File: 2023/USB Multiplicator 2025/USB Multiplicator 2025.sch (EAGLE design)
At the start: 11 parts, among them X1 USB-A

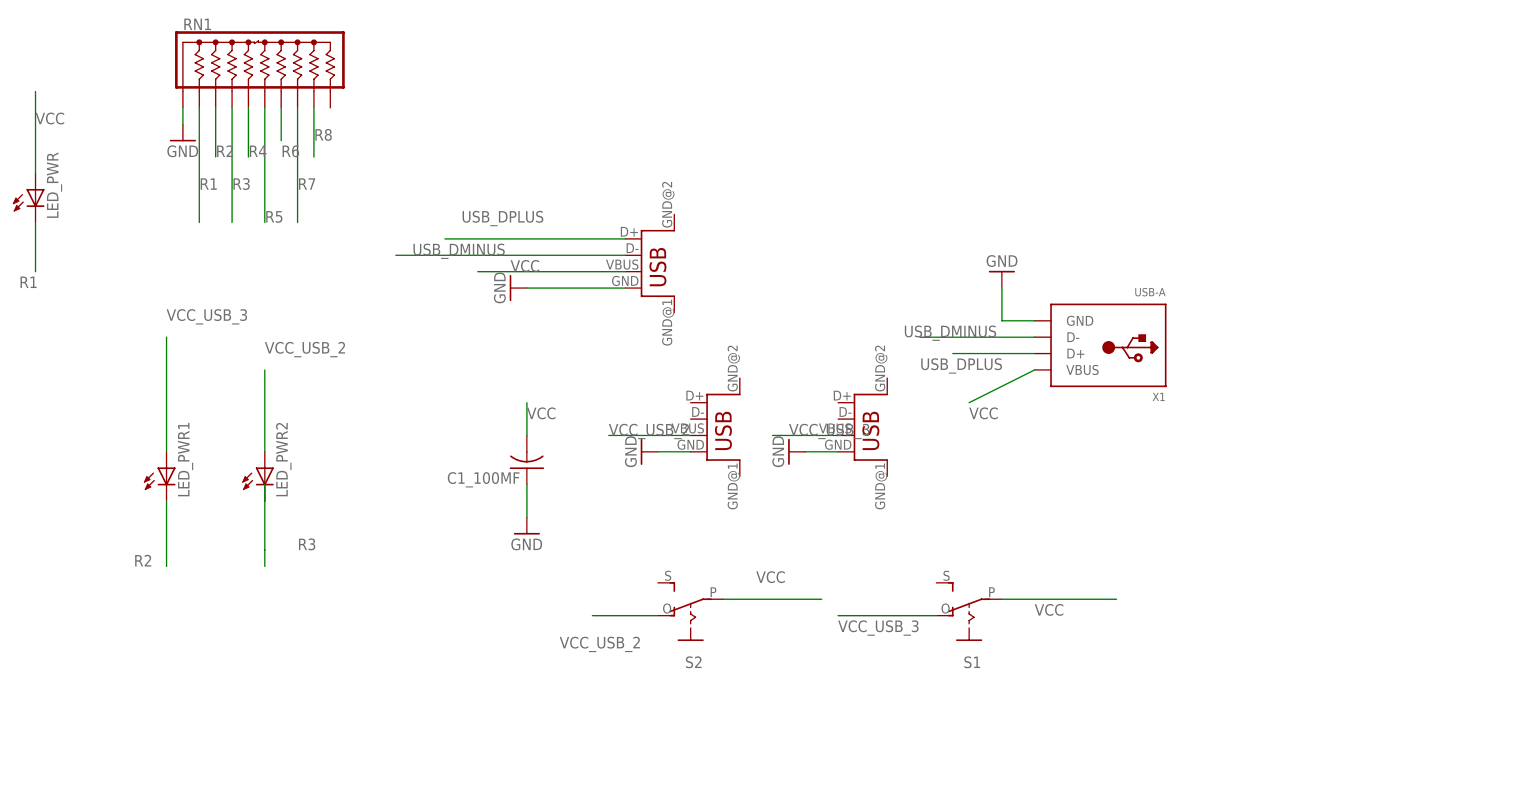
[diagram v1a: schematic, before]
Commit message: Update...
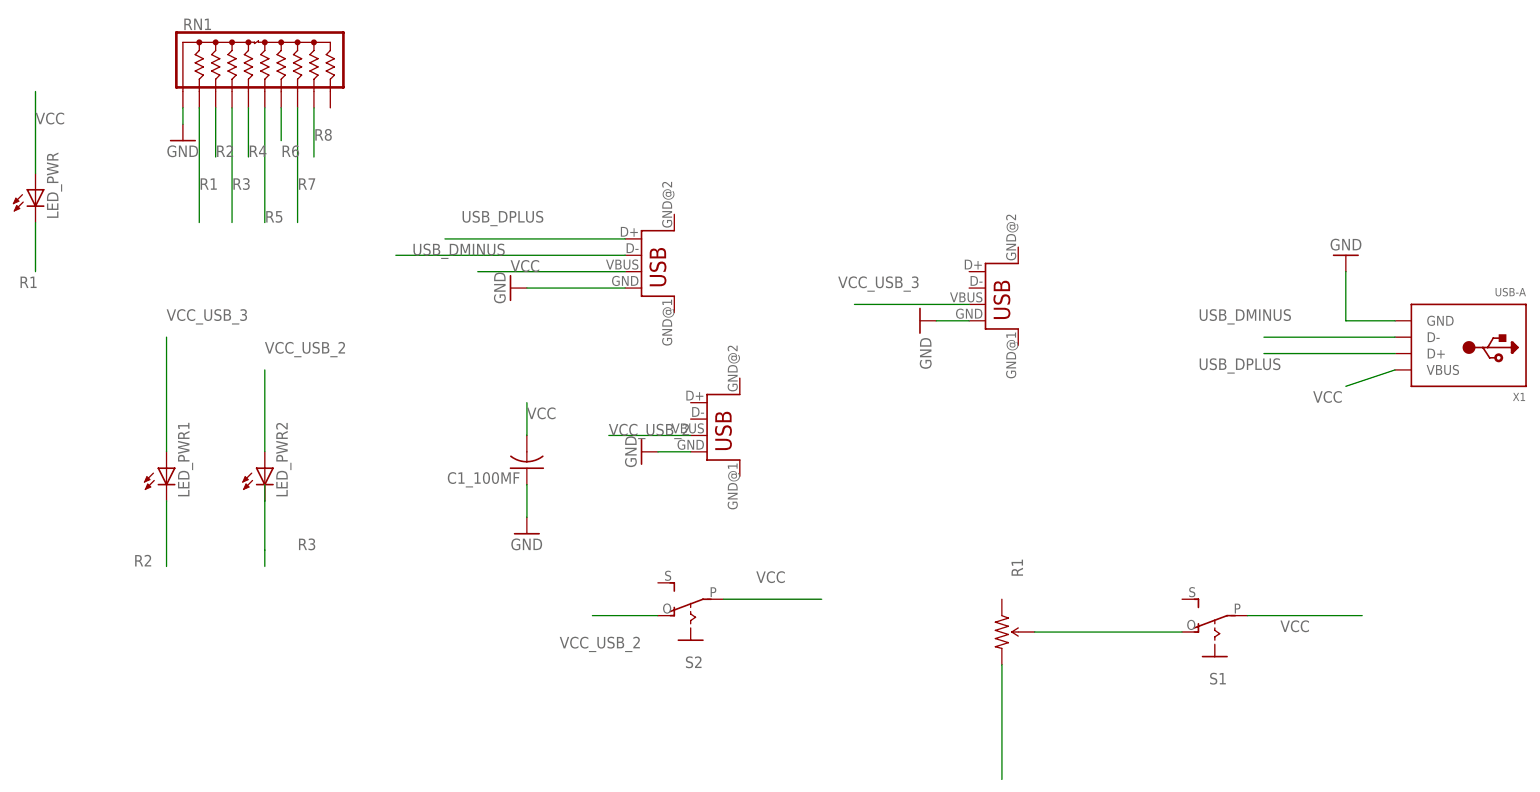
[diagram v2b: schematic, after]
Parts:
- added R1: (no value), SparkFun-Retired:TRIMPOTPTH
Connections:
- new net N$1: R1.WIPER, S1.O
- net VCC_USB_3: now also R1.CW; no longer S1.O
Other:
- moved on the sheet: S1, X1
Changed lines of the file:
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@@
 <layer number="56" name="wert" color="7" fill="1" visible="no" active="no"/>
 <layer number="57" name="tCAD" color="7" fill="1" visible="no" active="no"/>
+<layer number="59" name="tCarbon" color="7" fill="1" visible="no" active="no"/>
+<layer number="60" name="bCarbon" color="7" fill="1" visible="no" active="no"/>
+<layer number="88" name="SimResults" color="9" fill="1" visible="yes" active="yes"/>
+<layer number="89" name="SimProbes" color="9" fill="1" visible="yes" active="yes"/>
 <layer number="90" name="Modules" color="5" fill="1" visible="yes" active="yes"/>
 <layer number="91" name="Nets" color="2" fill="1" visible="yes" active="yes"/>
@@
 <layer number="112" name="tSilk" color="7" fill="1" visible="no" active="yes"/>
 <layer number="113" name="ReferenceLS" color="7" fill="1" visible="no" active="no"/>
+<layer number="114" name="Badge_Outline" color="11" fill="1" visible="no" active="no"/>
+<layer number="115" name="ReferenceISLANDS" color="7" fill="1" visible="yes" active="yes"/>
 <layer number="116" name="Patch_BOT" color="9" fill="4" visible="no" active="yes"/>
 <layer number="118" name="Rect_Pads" color="7" fill="1" visible="no" active="no"/>
@@
 <layer number="127" name="_tValues" color="7" fill="1" visible="no" active="yes"/>
 <layer number="128" name="_bValues" color="7" fill="1" visible="no" active="yes"/>
+<layer number="129" name="Mask" color="7" fill="1" visible="yes" active="yes"/>
 <layer number="131" name="tAdjust" color="7" fill="1" visible="no" active="yes"/>
 <layer number="132" name="bAdjust" color="7" fill="1" visible="no" active="yes"/>
@@
 <layer number="251" name="SMDround" color="7" fill="1" visible="no" active="no"/>
 <layer number="254" name="cooling" color="7" fill="1" visible="no" active="yes"/>
+<layer number="255" name="routoute" color="7" fill="1" visible="yes" active="yes"/>
 </layers>
 <schematic xreflabel="%F%N/%S.%C%R" xrefpart="/%S.%C%R">
@@
 <part name="RN1" library="resistor-sip" deviceset="4610X" device=""/>
 <part name="GND9" library="supply1" deviceset="GND" device=""/>
+<part name="R1" library="SparkFun-Retired" deviceset="TRIMPOT" device="PTH"/>
 </parts>
 <sheets>
@@
 </plain>
 <instances>
-<instance part="X1" gate="G$1" x="127" y="99.06" smashed="yes" rot="R180">
-<attribute name="NAME" x="137.16" y="90.424" size="1.27" layer="95" rot="R180"/>
-<attribute name="VALUE" x="137.16" y="106.68" size="1.27" layer="96" rot="R180"/>
-</instance>
-<instance part="GND1" gate="1" x="111.76" y="109.22" smashed="yes" rot="R180">
-<attribute name="VALUE" x="114.3" y="111.76" size="1.778" layer="96" rot="R180"/>
+<instance part="X1" gate="G$1" x="182.88" y="99.06" smashed="yes" rot="R180">
+<attribute name="NAME" x="193.04" y="90.424" size="1.27" layer="95" rot="R180"/>
+<attribute name="VALUE" x="193.04" y="106.68" size="1.27" layer="96" rot="R180"/>
+</instance>
+<instance part="GND1" gate="1" x="165.1" y="111.76" smashed="yes" rot="R180">
+<attribute name="VALUE" x="167.64" y="114.3" size="1.778" layer="96" rot="R180"/>
 </instance>
 <instance part="C1_100MF" gate="G$1" x="38.1" y="78.74" smashed="yes" rot="R180">
@@
 </instance>
 <instance part="USB_OUT_2" gate="G$1" x="66.04" y="78.74" smashed="yes"/>
-<instance part="USB_OUT_3" gate="G$1" x="88.9" y="78.74" smashed="yes"/>
+<instance part="USB_OUT_3" gate="G$1" x="109.22" y="99.06" smashed="yes"/>
 <instance part="GND3" gate="1" x="55.88" y="81.28" smashed="yes" rot="R270">
 <attribute name="VALUE" x="53.34" y="83.82" size="1.778" layer="96" rot="R270"/>
 </instance>
-<instance part="GND4" gate="1" x="78.74" y="81.28" smashed="yes" rot="R270">
-<attribute name="VALUE" x="76.2" y="83.82" size="1.778" layer="96" rot="R270"/>
+<instance part="GND4" gate="1" x="99.06" y="101.6" smashed="yes" rot="R270">
+<attribute name="VALUE" x="99.06" y="99.06" size="1.778" layer="96" rot="R270"/>
 </instance>
 <instance part="S2" gate="1" x="63.5" y="55.88" smashed="yes" rot="R90">
@@
 <attribute name="VALUE" x="60.325" y="52.07" size="1.778" layer="96" rot="R180"/>
 </instance>
-<instance part="S1" gate="1" x="106.68" y="55.88" smashed="yes" rot="R90">
-<attribute name="NAME" x="108.585" y="49.53" size="1.778" layer="95" rot="R180"/>
-<attribute name="VALUE" x="103.505" y="52.07" size="1.778" layer="96" rot="R180"/>
+<instance part="S1" gate="1" x="144.78" y="53.34" smashed="yes" rot="R90">
+<attribute name="NAME" x="146.685" y="46.99" size="1.778" layer="95" rot="R180"/>
+<attribute name="VALUE" x="141.605" y="49.53" size="1.778" layer="96" rot="R180"/>
 </instance>
 <instance part="LED_PWR2" gate="G$1" x="-2.54" y="78.74" smashed="yes">
@@
 <instance part="GND9" gate="1" x="-15.24" y="129.54" smashed="yes">
 <attribute name="VALUE" x="-17.78" y="127" size="1.778" layer="96"/>
+</instance>
+<instance part="R1" gate="R?" x="111.76" y="53.34" smashed="yes" rot="R270">
+<attribute name="NAME" x="113.2586" y="64.77" size="1.778" layer="95" rot="R270"/>
+<attribute name="VALUE" x="108.458" y="57.15" size="1.778" layer="96" rot="R270"/>
 </instance>
 </instances>
@@
 <segment>
 <pinref part="X1" gate="G$1" pin="GND"/>
-<wire x1="116.84" y1="101.6" x2="111.76" y2="101.6" width="0.1524" layer="91"/>
+<wire x1="172.72" y1="101.6" x2="165.1" y2="101.6" width="0.1524" layer="91"/>
 <pinref part="GND1" gate="1" pin="GND"/>
-<wire x1="111.76" y1="101.6" x2="111.76" y2="106.68" width="0.1524" layer="91"/>
+<wire x1="165.1" y1="101.6" x2="165.1" y2="109.22" width="0.1524" layer="91"/>
 </segment>
 <segment>
@@
 <pinref part="GND4" gate="1" pin="GND"/>
 <pinref part="USB_OUT_3" gate="G$1" pin="GND"/>
-<wire x1="81.28" y1="81.28" x2="86.36" y2="81.28" width="0.1524" layer="91"/>
+<wire x1="101.6" y1="101.6" x2="106.68" y2="101.6" width="0.1524" layer="91"/>
 </segment>
 <segment>
@@
 <segment>
 <pinref part="X1" gate="G$1" pin="VBUS"/>
-<wire x1="116.84" y1="93.98" x2="106.68" y2="88.9" width="0.1524" layer="91"/>
-<label x="106.68" y="86.36" size="1.778" layer="95"/>
+<wire x1="172.72" y1="93.98" x2="165.1" y2="91.44" width="0.1524" layer="91"/>
+<label x="160.02" y="88.9" size="1.778" layer="95"/>
 </segment>
 <segment>
 <pinref part="S1" gate="1" pin="P"/>
-<wire x1="111.76" y1="58.42" x2="129.54" y2="58.42" width="0.1524" layer="91"/>
-<label x="116.84" y="55.88" size="1.778" layer="95"/>
+<wire x1="149.86" y1="55.88" x2="167.64" y2="55.88" width="0.1524" layer="91"/>
+<label x="154.94" y="53.34" size="1.778" layer="95"/>
 </segment>
 </net>
@@
 <segment>
 <pinref part="X1" gate="G$1" pin="D+"/>
-<wire x1="116.84" y1="96.52" x2="104.14" y2="96.52" width="0.1524" layer="91"/>
-<label x="99.06" y="93.98" size="1.778" layer="95"/>
+<wire x1="172.72" y1="96.52" x2="152.4" y2="96.52" width="0.1524" layer="91"/>
+<label x="142.24" y="93.98" size="1.778" layer="95"/>
 </segment>
 <segment>
@@
 <segment>
 <pinref part="X1" gate="G$1" pin="D-"/>
-<wire x1="116.84" y1="99.06" x2="99.06" y2="99.06" width="0.1524" layer="91"/>
-<label x="96.52" y="99.06" size="1.778" layer="95"/>
+<wire x1="172.72" y1="99.06" x2="152.4" y2="99.06" width="0.1524" layer="91"/>
+<label x="142.24" y="101.6" size="1.778" layer="95"/>
 </segment>
 <segment>
@@
 <segment>
 <pinref part="USB_OUT_3" gate="G$1" pin="VBUS"/>
-<wire x1="86.36" y1="83.82" x2="76.2" y2="83.82" width="0.1524" layer="91"/>
-<label x="78.74" y="83.82" size="1.778" layer="95"/>
-</segment>
-<segment>
-<pinref part="S1" gate="1" pin="O"/>
-<wire x1="101.6" y1="55.88" x2="86.36" y2="55.88" width="0.1524" layer="91"/>
-<label x="86.36" y="53.34" size="1.778" layer="95"/>
+<wire x1="106.68" y1="104.14" x2="88.9" y2="104.14" width="0.1524" layer="91"/>
+<label x="86.36" y="106.68" size="1.778" layer="95"/>
 </segment>
 <segment>
@@
 <wire x1="-17.78" y1="81.28" x2="-17.78" y2="99.06" width="0.1524" layer="91"/>
 <label x="-17.78" y="101.6" size="1.778" layer="95"/>
+</segment>
+<segment>
+<pinref part="R1" gate="R?" pin="CW"/>
+<wire x1="111.76" y1="48.26" x2="111.76" y2="30.48" width="0.1524" layer="91"/>
 </segment>
 </net>
@@
 </segment>
 </net>
+<net name="N$1" class="0">
+<segment>
+<pinref part="S1" gate="1" pin="O"/>
+<pinref part="R1" gate="R?" pin="WIPER"/>
+<wire x1="139.7" y1="53.34" x2="116.84" y2="53.34" width="0.1524" layer="91"/>
+</segment>
+</net>

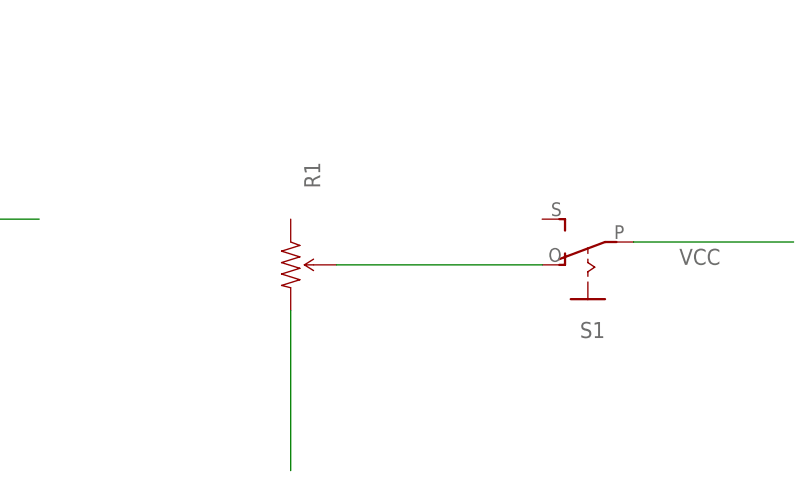
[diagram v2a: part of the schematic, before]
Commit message: Update...
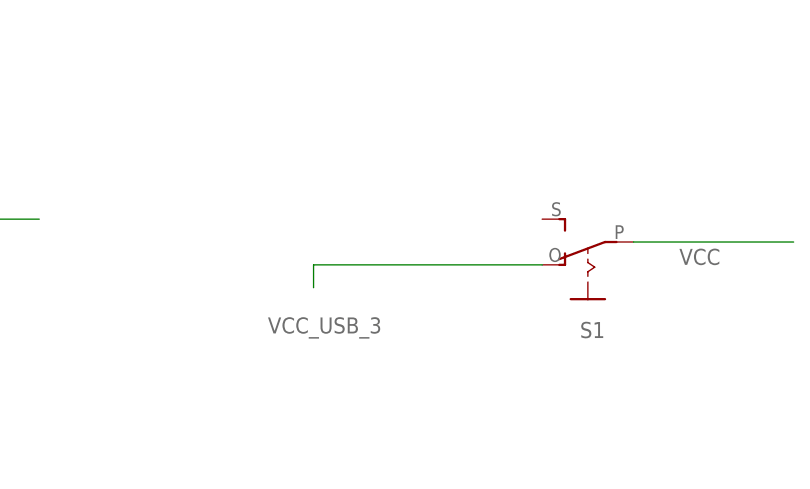
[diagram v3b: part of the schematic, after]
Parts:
- removed R1: (no value), SparkFun-Retired:TRIMPOTPTH
- renumbered USB_OUT_3 to USB_OUT_1
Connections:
- removed net N$1: R1.WIPER, S1.O
- net VCC_USB_3: now also S1.O; no longer R1.CW
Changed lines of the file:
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@@
 <part name="GND2" library="supply1" deviceset="GND" device=""/>
 <part name="USB_OUT_2" library="STUNTAZ" deviceset="USB" device=""/>
-<part name="USB_OUT_3" library="STUNTAZ" deviceset="USB" device=""/>
+<part name="USB_OUT_1" library="STUNTAZ" deviceset="USB" device=""/>
 <part name="GND3" library="supply1" deviceset="GND" device=""/>
 <part name="GND4" library="supply1" deviceset="GND" device=""/>
@@
 <part name="RN1" library="resistor-sip" deviceset="4610X" device=""/>
 <part name="GND9" library="supply1" deviceset="GND" device=""/>
-<part name="R1" library="SparkFun-Retired" deviceset="TRIMPOT" device="PTH"/>
 </parts>
 <sheets>
@@
 </instance>
 <instance part="USB_OUT_2" gate="G$1" x="66.04" y="78.74" smashed="yes"/>
-<instance part="USB_OUT_3" gate="G$1" x="109.22" y="99.06" smashed="yes"/>
+<instance part="USB_OUT_1" gate="G$1" x="109.22" y="99.06" smashed="yes"/>
 <instance part="GND3" gate="1" x="55.88" y="81.28" smashed="yes" rot="R270">
 <attribute name="VALUE" x="53.34" y="83.82" size="1.778" layer="96" rot="R270"/>
@@
 <instance part="GND9" gate="1" x="-15.24" y="129.54" smashed="yes">
 <attribute name="VALUE" x="-17.78" y="127" size="1.778" layer="96"/>
-</instance>
-<instance part="R1" gate="R?" x="111.76" y="53.34" smashed="yes" rot="R270">
-<attribute name="NAME" x="113.2586" y="64.77" size="1.778" layer="95" rot="R270"/>
-<attribute name="VALUE" x="108.458" y="57.15" size="1.778" layer="96" rot="R270"/>
 </instance>
 </instances>
@@
 <segment>
 <pinref part="GND4" gate="1" pin="GND"/>
-<pinref part="USB_OUT_3" gate="G$1" pin="GND"/>
+<pinref part="USB_OUT_1" gate="G$1" pin="GND"/>
 <wire x1="101.6" y1="101.6" x2="106.68" y2="101.6" width="0.1524" layer="91"/>
 </segment>
@@
 <net name="VCC_USB_3" class="0">
 <segment>
-<pinref part="USB_OUT_3" gate="G$1" pin="VBUS"/>
+<pinref part="USB_OUT_1" gate="G$1" pin="VBUS"/>
 <wire x1="106.68" y1="104.14" x2="88.9" y2="104.14" width="0.1524" layer="91"/>
 <label x="86.36" y="106.68" size="1.778" layer="95"/>
@@
 </segment>
 <segment>
-<pinref part="R1" gate="R?" pin="CW"/>
-<wire x1="111.76" y1="48.26" x2="111.76" y2="30.48" width="0.1524" layer="91"/>
+<pinref part="S1" gate="1" pin="O"/>
+<wire x1="139.7" y1="53.34" x2="114.3" y2="53.34" width="0.1524" layer="91"/>
+<wire x1="114.3" y1="53.34" x2="114.3" y2="50.8" width="0.1524" layer="91"/>
+<label x="109.22" y="45.72" size="1.778" layer="95"/>
 </segment>
 </net>
@@
 </segment>
 </net>
-<net name="N$1" class="0">
-<segment>
-<pinref part="S1" gate="1" pin="O"/>
-<pinref part="R1" gate="R?" pin="WIPER"/>
-<wire x1="139.7" y1="53.34" x2="116.84" y2="53.34" width="0.1524" layer="91"/>
-</segment>
-</net>
